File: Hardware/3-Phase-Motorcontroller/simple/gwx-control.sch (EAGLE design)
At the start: 23 parts, among them IC1 74LS02D, IC2 74LS123D

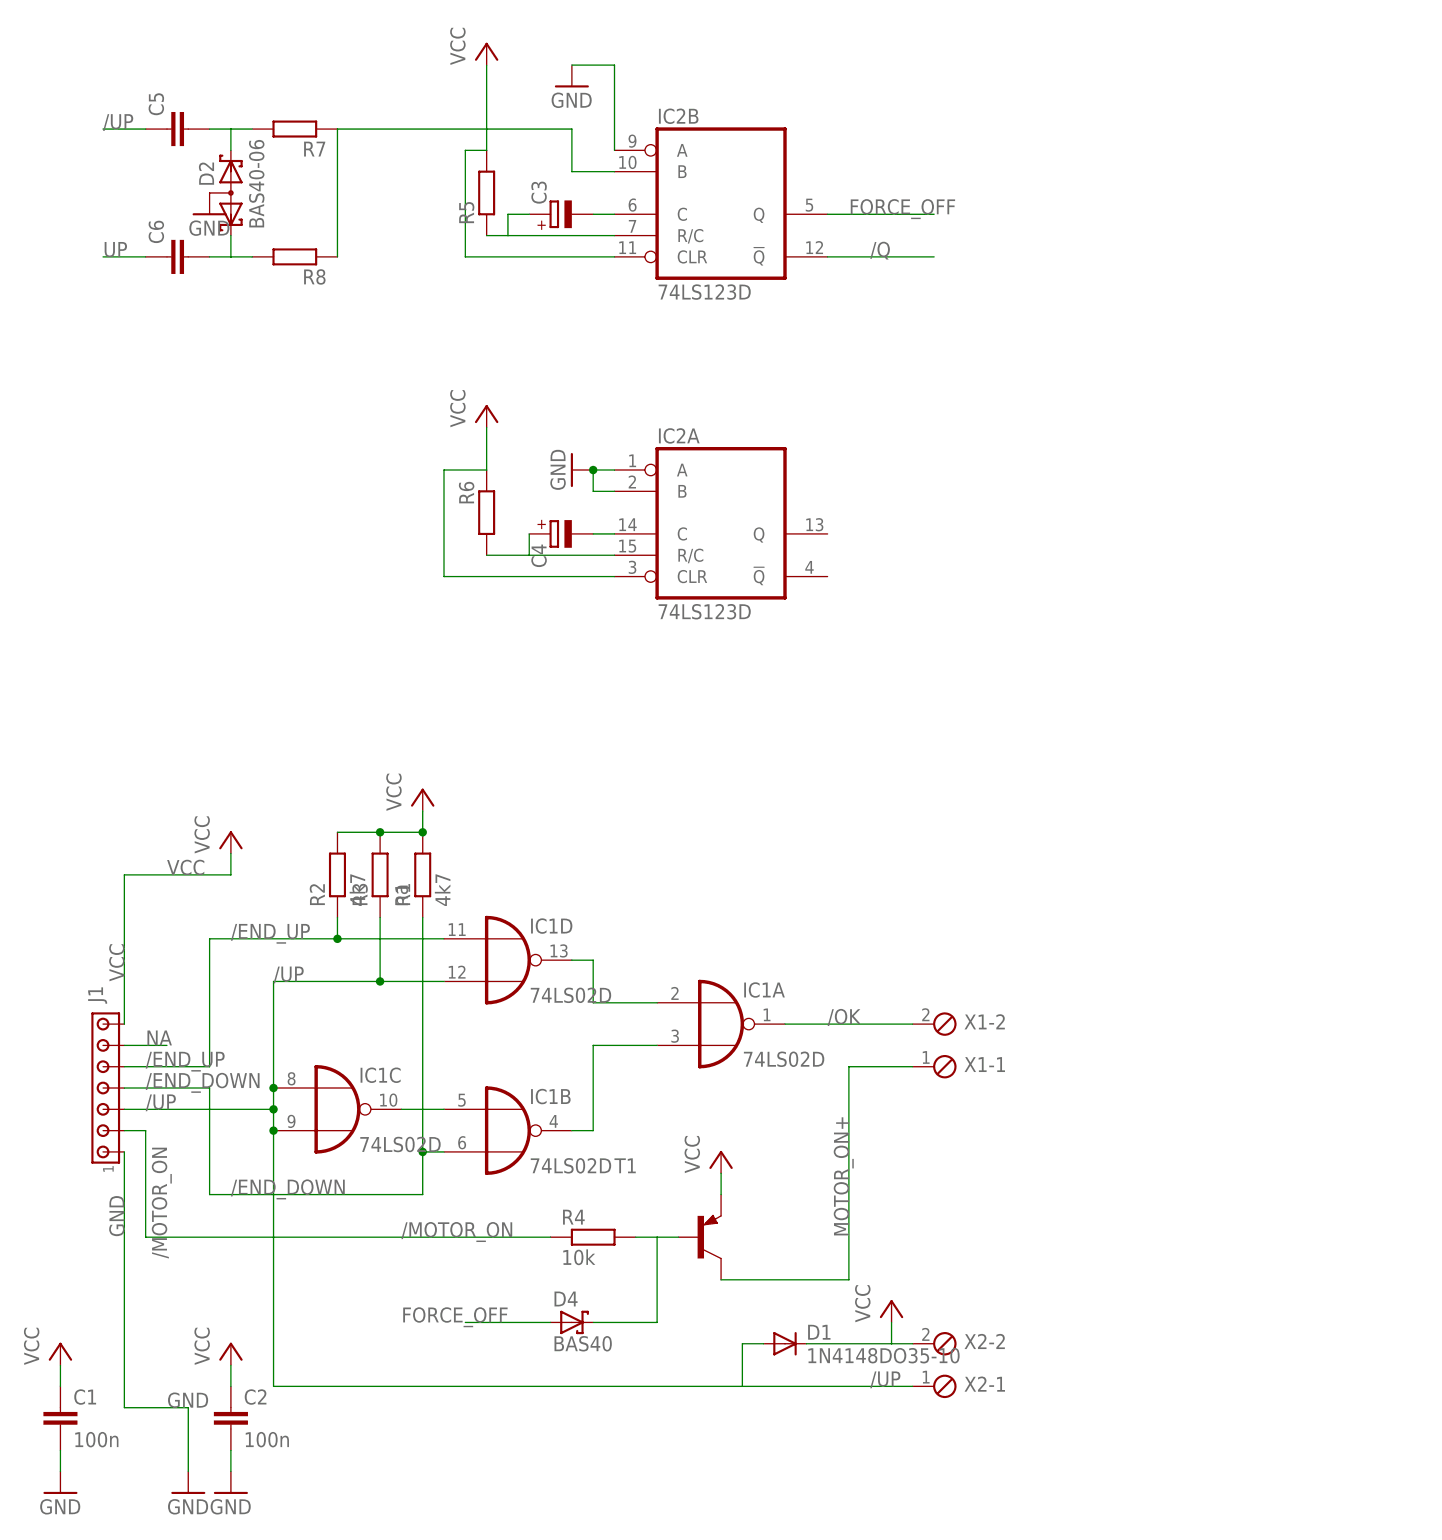
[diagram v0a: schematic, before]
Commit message: Trigger fixed
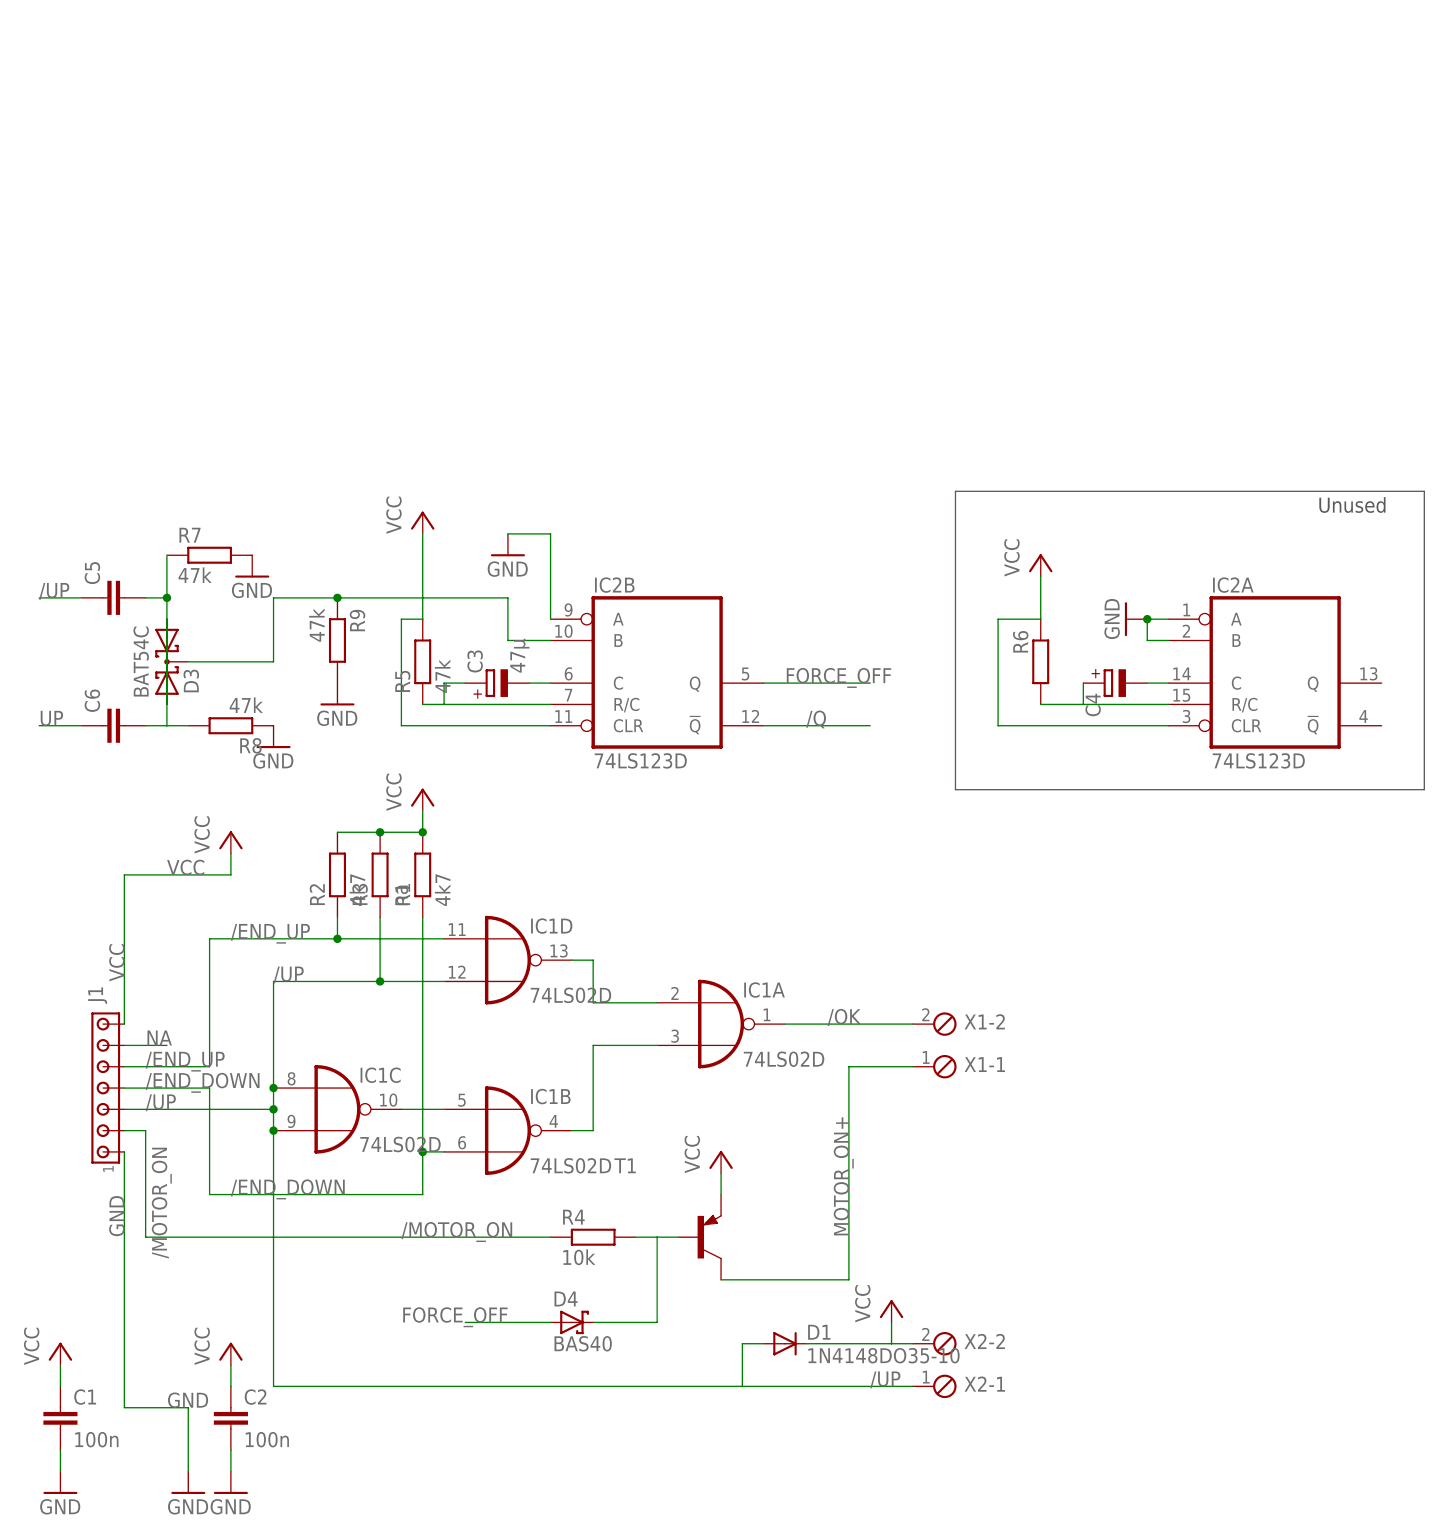
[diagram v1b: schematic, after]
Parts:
- removed D2: BAS40-06, diode:BAS40-06
- added D3: BAT54C, diode:BAT54C
- added R9: 47k, rcl:R-EU_R0603
- C3: value (none) -> 47µ
- R5, R7, R8: value (none) -> 47k
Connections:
- net GND: now also R7.2, R8.1, R9.2; no longer D2.AA
- net N$4: now also D3.A2, R7.1; no longer D2.K2, R7.2
- net N$7: now also D3.A1; no longer D2.K1
- net N$8: now also D3.CC, R9.1; no longer R7.1, R8.1
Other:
- note added: "Unused"
- moved on the sheet: C3, C4, C5, C6, IC2A, IC2B, R5, R6, R7, R8
